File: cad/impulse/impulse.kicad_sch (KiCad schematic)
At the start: 0 parts

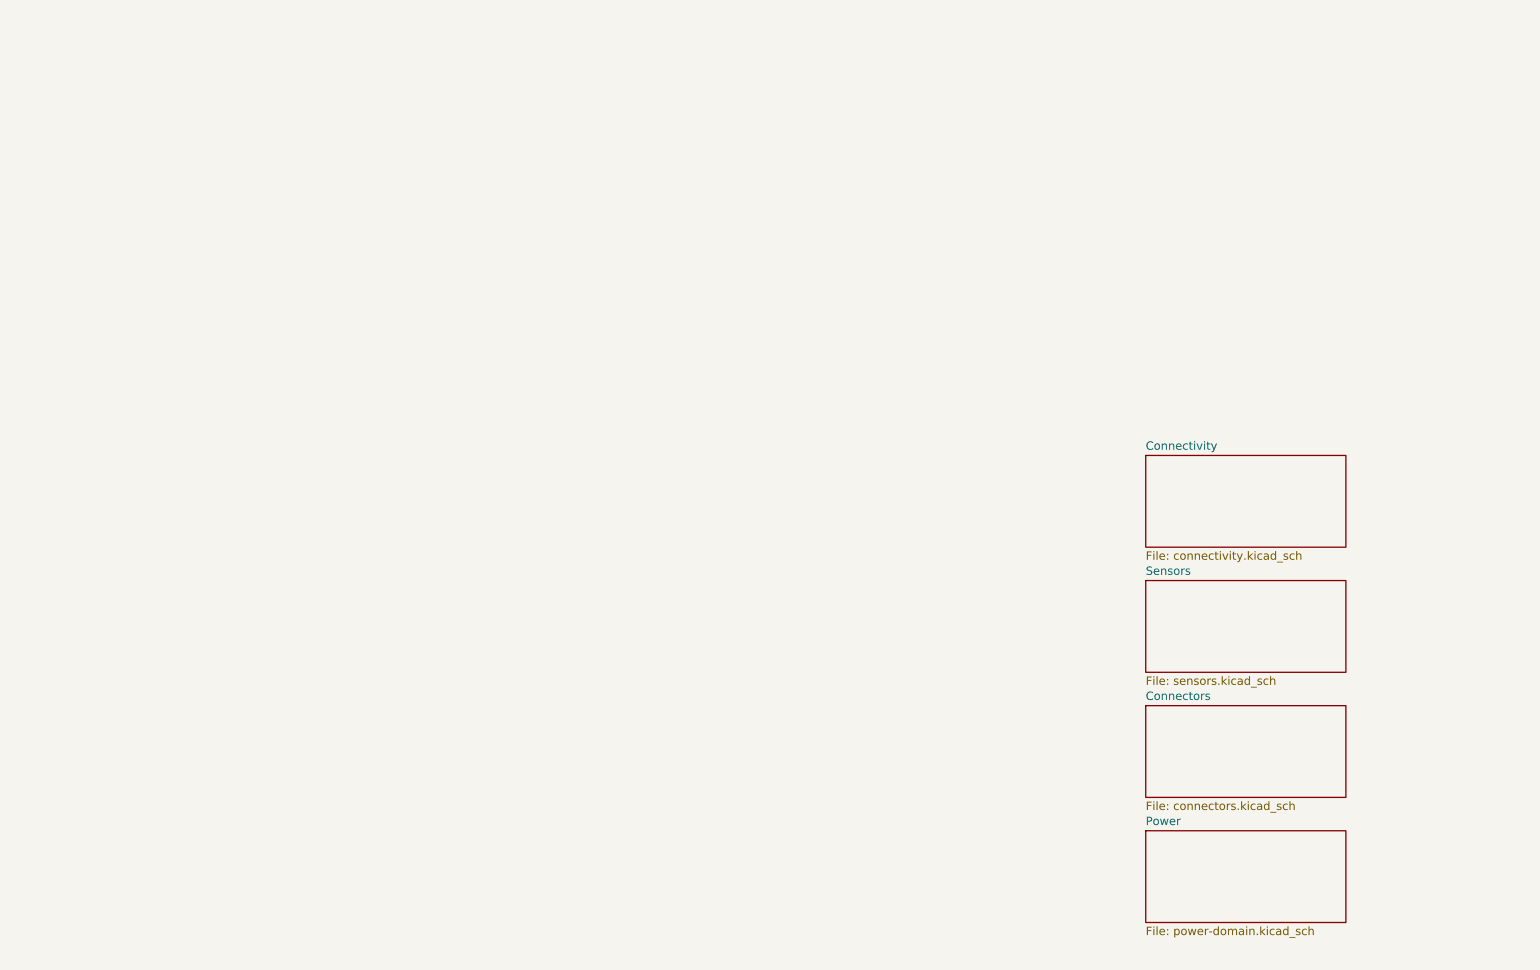
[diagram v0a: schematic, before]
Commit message: Finnished the design.
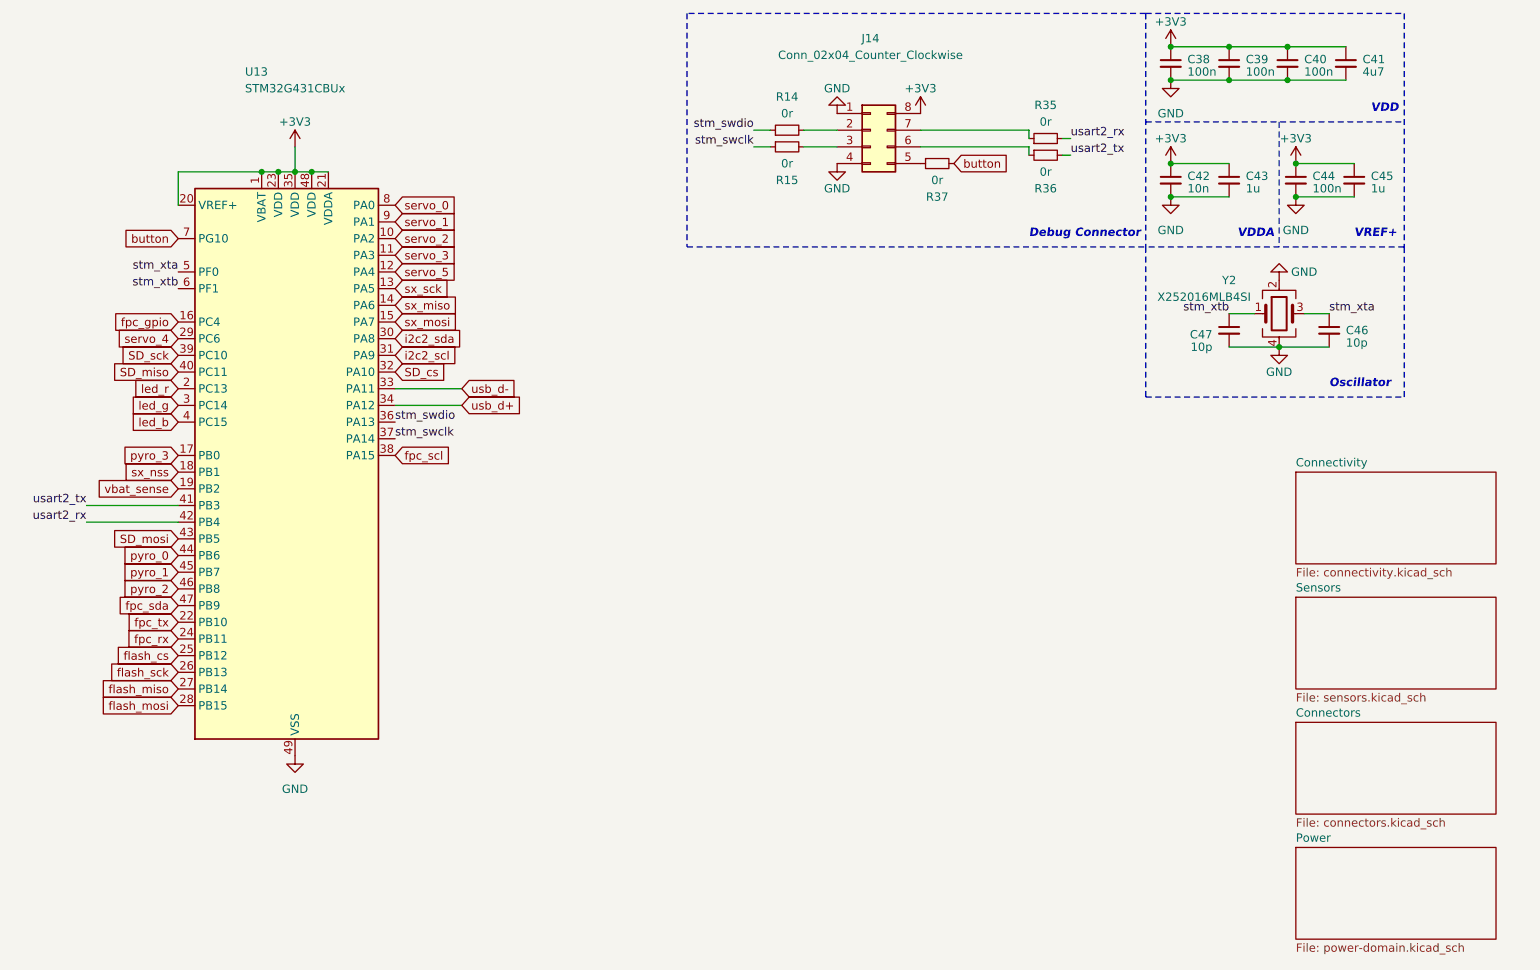
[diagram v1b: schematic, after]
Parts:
- added C38, C39, C40, C44: 100n, symbol Device:C_Small
- added C41: 4u7, symbol Device:C_Small
- added C42: 10n, symbol Device:C_Small
- added C43, C45: 1u, symbol Device:C_Small
- added C46, C47: 10p, symbol Device:C_Small
- added J14: Conn_02x04_Counter_Clockwise, symbol Connector_Generic:Conn_02x04_Counter_Clockwise
- added R14, R15, R35, R36, R37: 0r, symbol Device:R_Small
- added U13: STM32G431CBUx, symbol MCU_ST_STM32G4:STM32G431CBUx
- added Y2: X252016MLB4SI, symbol Device:Crystal_GND24
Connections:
- new net: J14.2 (Pin_2), R14.2
- new net: J14.3 (Pin_3), R15.2
- new net: J14.5 (Pin_5), R37.1
- new net: J14.6 (Pin_6), R36.1
- new net: J14.7 (Pin_7), R35.1
- new net +3V3: C38.1, C39.1, C40.1, C41.1, C42.1, C43.1, C44.1, C45.1, J14.8 (Pin_8), U13.1 (VBAT), U13.20 (VREF+), U13.21 (VDDA), U13.23 (VDD), U13.35 (VDD), U13.48 (VDD)
- new net GND: C38.2, C39.2, C40.2, C41.2, C42.2, C43.2, C44.2, C45.2, C46.2, C47.2, J14.1 (Pin_1), J14.4 (Pin_4), U13.49 (VSS), Y2.2, Y2.4
- new net SD_cs: U13.32 (PA10)
- new net SD_miso: U13.40 (PC11)
- new net SD_mosi: U13.43 (PB5)
- new net SD_sck: U13.39 (PC10)
- new net button: R37.2, U13.7 (PG10)
- new net flash_cs: U13.25 (PB12)
- new net flash_miso: U13.27 (PB14)
- new net flash_mosi: U13.28 (PB15)
- new net flash_sck: U13.26 (PB13)
- new net fpc_gpio: U13.16 (PC4)
- new net fpc_rx: U13.24 (PB11)
- new net fpc_scl: U13.38 (PA15)
- new net fpc_sda: U13.47 (PB9)
- new net fpc_tx: U13.22 (PB10)
- new net i2c2_scl: U13.31 (PA9)
- new net i2c2_sda: U13.30 (PA8)
- new net led_b: U13.4 (PC15)
- new net led_g: U13.3 (PC14)
- new net led_r: U13.2 (PC13)
- new net pyro_0: U13.44 (PB6)
- new net pyro_1: U13.45 (PB7)
- new net pyro_2: U13.46 (PB8)
- new net pyro_3: U13.17 (PB0)
- new net servo_0: U13.8 (PA0)
- new net servo_1: U13.9 (PA1)
- new net servo_2: U13.10 (PA2)
- new net servo_3: U13.11 (PA3)
- new net servo_4: U13.29 (PC6)
- new net servo_5: U13.12 (PA4)
- new net stm_swclk: R15.1, U13.37 (PA14)
- new net stm_swdio: R14.1, U13.36 (PA13)
- new net stm_xta: C46.1, U13.5 (PF0), Y2.3
- new net stm_xtb: C47.1, U13.6 (PF1), Y2.1
- new net sx_miso: U13.14 (PA6)
- new net sx_mosi: U13.15 (PA7)
- new net sx_nss: U13.18 (PB1)
- new net sx_sck: U13.13 (PA5)
- new net usart2_rx: R35.2, U13.42 (PB4)
- new net usart2_tx: R36.2, U13.41 (PB3)
- new net usb_d+: U13.34 (PA12)
- new net usb_d-: U13.33 (PA11)
- new net vbat_sense: U13.19 (PB2)
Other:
- note added: "Debug Connector"
- note added: "Oscillator"
- note added: "VDD"
- note added: "VDDA"
- note added: "VREF+"
- company: (none) -> markbel
- title: (none) -> MCU
